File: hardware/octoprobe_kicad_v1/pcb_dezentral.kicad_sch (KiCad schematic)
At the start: 63 parts, among them J1 weidmueller_SL5.08HC-06-90, J2 weidmueller_SL5.08HC-10-90, Q1 AO3400A, SW1 dip_switch_SPST16, U1 SP3485EN-L/TR, U2 AOZ1282CI

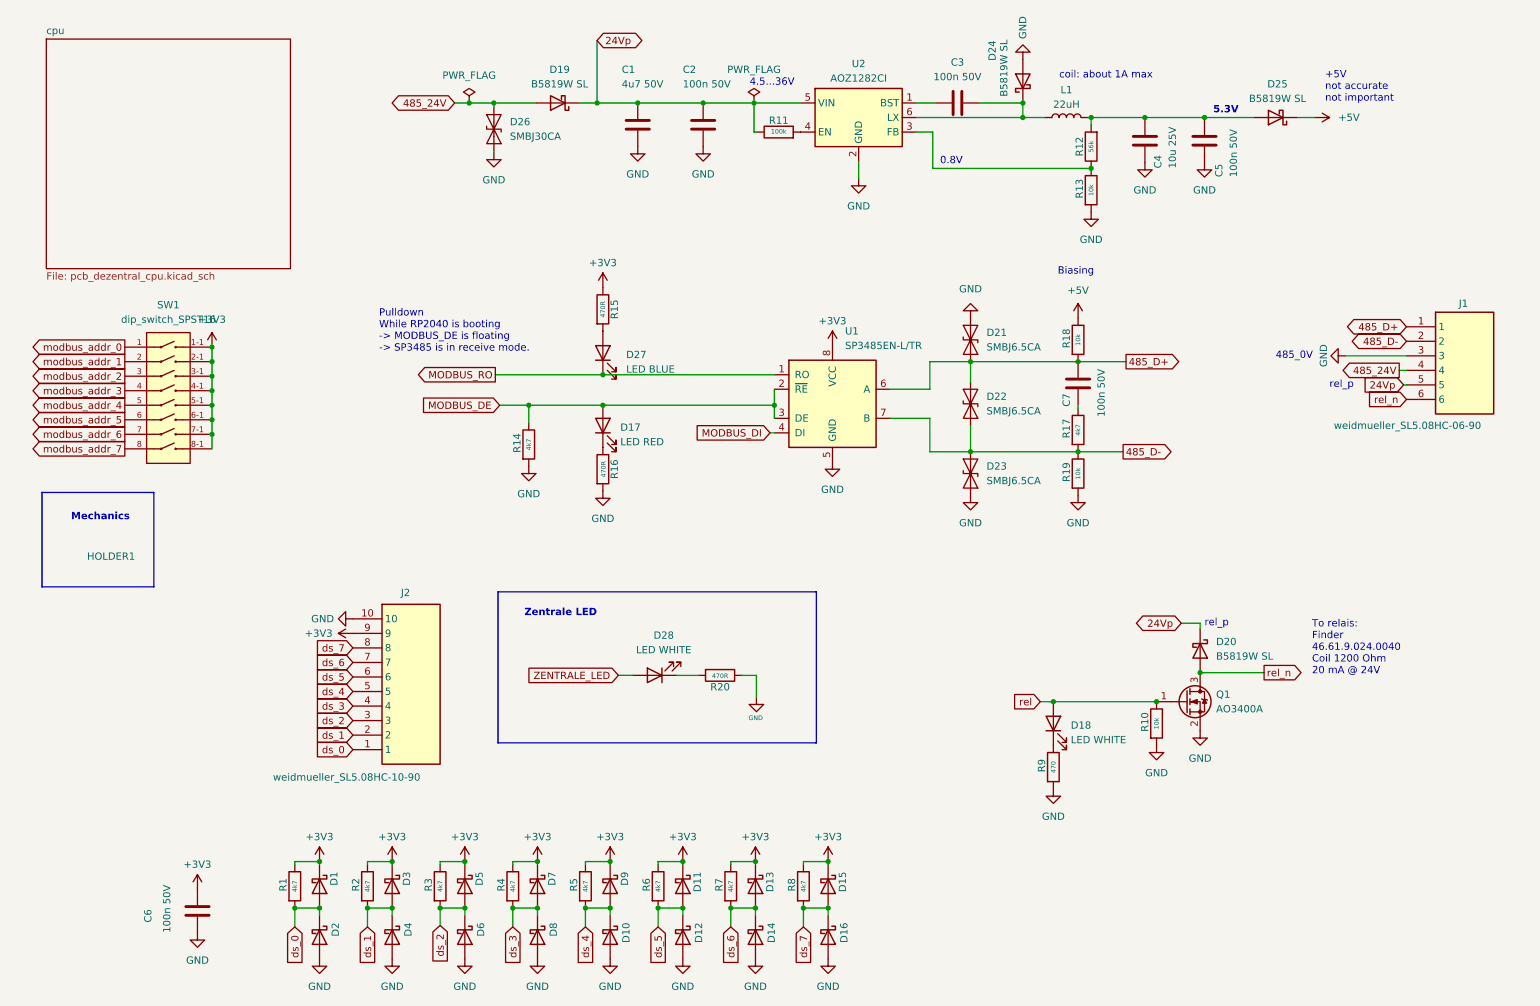
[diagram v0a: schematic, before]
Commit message: cleanup pcb
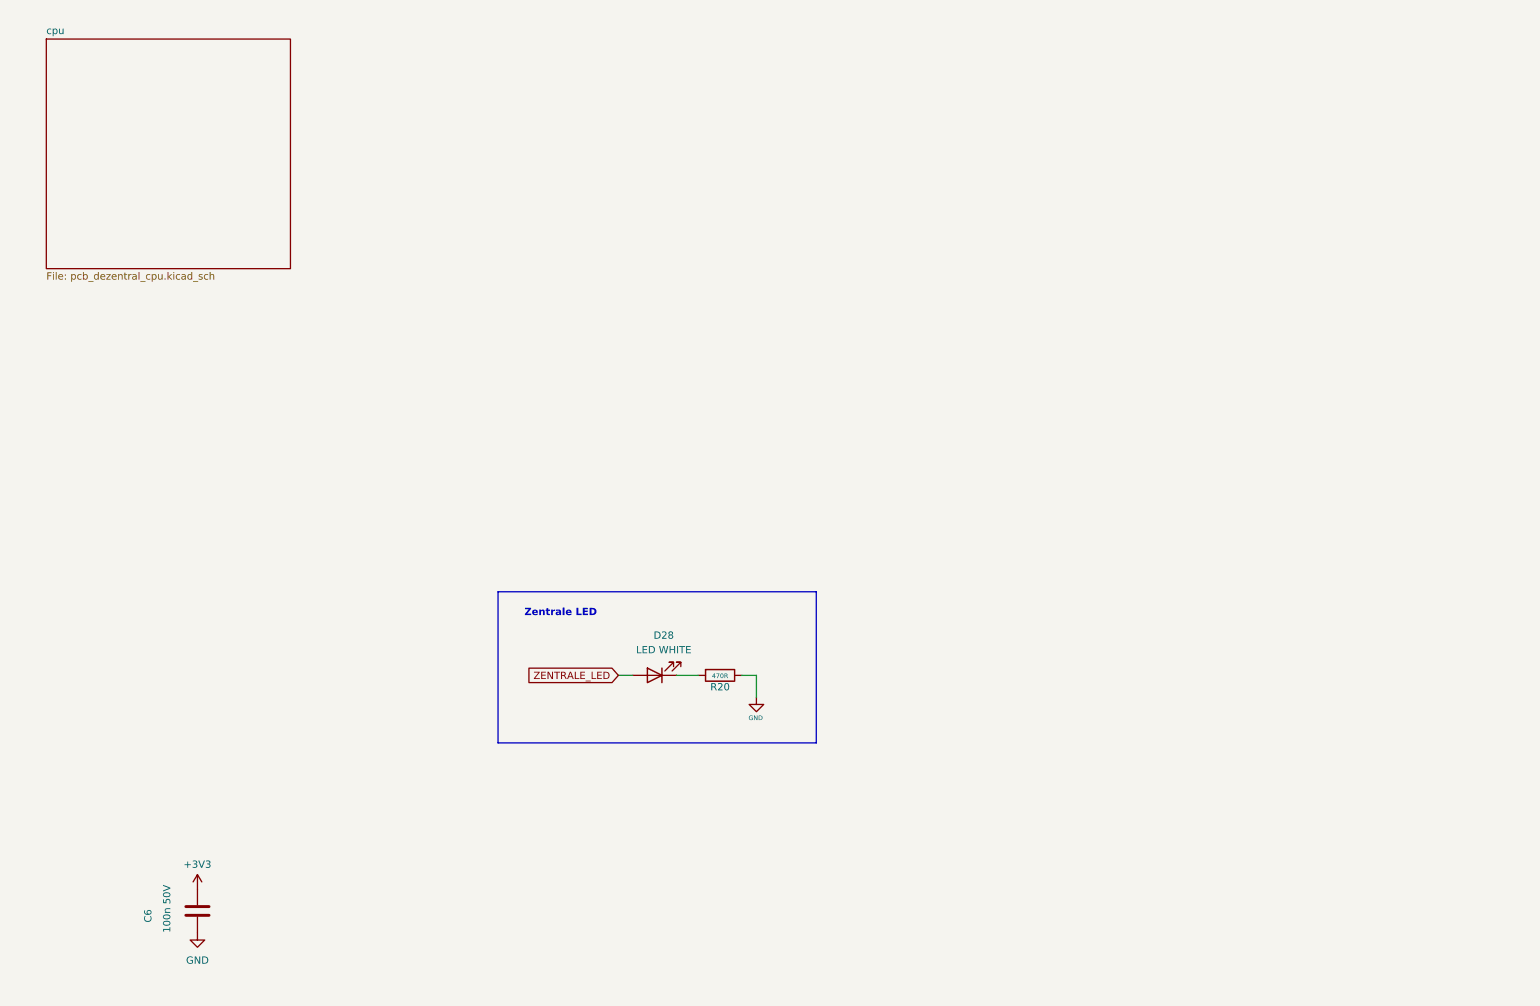
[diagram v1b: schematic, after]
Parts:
- removed C1: 4u7 50V, Diode_SMD:D_1206_3216Metric, symbol Device:C
- removed C2, C3, C5, C7: 100n 50V, Diode_SMD:D_0805_2012Metric, symbol Device:C
- removed C4: 10u 25V, Diode_SMD:D_0805_2012Metric, symbol Device:C
- removed D1, D10, D11, D12, D13, D14, D15, D16, D19, D2, D20, D24, D25, D3, D4, D5, D6, D7, D8, D9: B5819W SL, Diode_SMD:D_SOD-123, symbol Device:D_Schottky
- removed D17: LED RED, 00_project_library:LED_0603_1608Metric, symbol 00_project_library:LED RED
- removed D18: LED WHITE, 00_project_library:LED_0603_1608Metric, symbol 00_project_library:LED WHITE
- removed D21, D22, D23: SMBJ6.5CA, Diode_SMD:D_SMB, symbol Diode:SMAJ64CA
- removed D26: SMBJ30CA, Diode_SMD:D_SMB, symbol Diode:SMAJ64CA
- removed D27: LED BLUE, 00_project_library:LED_0603_1608Metric, symbol 00_project_library:LED BLUE
- removed J1: weidmueller_SL5.08HC-06-90, 00_project_library:weidmueller_SL5.08HC-06-90, symbol 00_project_library:weidmueller_SL5.08HC-06-90
- removed J2: weidmueller_SL5.08HC-10-90, 00_project_library:weidmueller_SL5.08HC-10-90, symbol 00_project_library:weidmueller_SL5.08HC-10-90
- removed L1: 22uH, 00_project_library:L_MODBUS, symbol Device:L
- removed Q1: AO3400A, Package_TO_SOT_SMD:SOT-23, symbol Transistor_FET:AO3400A
- removed R1, R14, R17, R2, R3, R4, R5, R6, R7, R8: 4k7, Resistor_SMD:R_0402_1005Metric_Pad0.72x0.64mm_HandSolder, symbol Device:R
- removed R10, R13, R18, R19: 10k, Resistor_SMD:R_0402_1005Metric_Pad0.72x0.64mm_HandSolder, symbol Device:R
- removed R11: 100k, Resistor_SMD:R_0402_1005Metric_Pad0.72x0.64mm_HandSolder, symbol Device:R
- removed R12: 56k, Resistor_SMD:R_0402_1005Metric_Pad0.72x0.64mm_HandSolder, symbol Device:R
- removed R15, R16: 470R, Resistor_SMD:R_0402_1005Metric_Pad0.72x0.64mm_HandSolder, symbol Device:R
- removed R9: 470, Resistor_SMD:R_0402_1005Metric_Pad0.72x0.64mm_HandSolder, symbol Device:R
- removed SW1: dip_switch_SPST16, 00_project_library:dip_switch_SPST16, symbol 00_project_library:dip_switch_SPST16
- removed U1: SP3485EN-L/TR, Package_SO:SOIC-8_3.9x4.9mm_P1.27mm, symbol 00_project_library:modbus_SP3485EN
- removed U2: AOZ1282CI, Package_TO_SOT_SMD:SOT-23-6, symbol Regulator_Switching:AOZ1282CI
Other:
- note removed: "+5V not accurate not important"
- note removed: "0.8V"
- note removed: "4.5...36V"
- note removed: "485_0V"
- note removed: "5.3V"
- note removed: "Biasing"
- note removed: "Mechanics"
- note removed: "Pulldown While RP2040 is booting -> MODBUS_DE is floating -> SP3485 is in receive mode."
- note removed: "To relais: Finder 46.61.9.024.0040 Coil 1200 Ohm 20 mA @ 24V"
- note removed: "coil: about 1A max"
- note removed: "rel_p"
